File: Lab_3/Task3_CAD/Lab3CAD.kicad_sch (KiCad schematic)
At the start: 25 parts, among them J1 Conn_01x02, T1 Transformer_1P_1S, T2 Transformer_1P_1S, U1 LM317_TO-220, U2 LM337_TO220

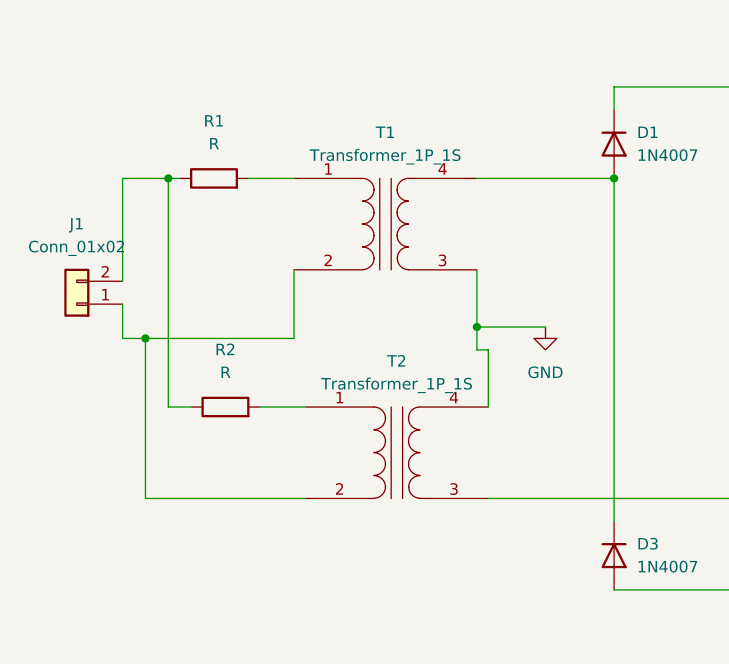
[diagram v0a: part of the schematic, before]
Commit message: block diagram
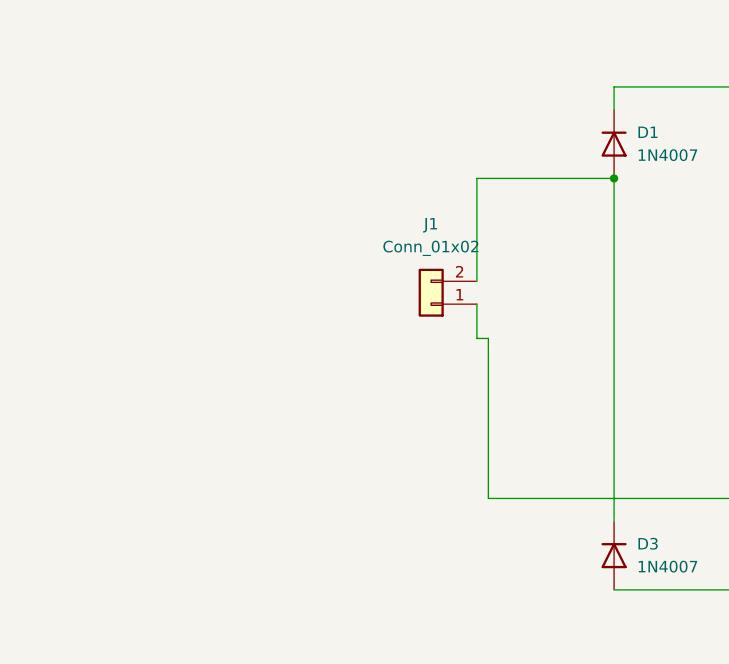
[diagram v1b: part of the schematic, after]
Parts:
- removed R1, R2: R, Resistor_THT:R_Axial_DIN0207_L6.3mm_D2.5mm_P7.62mm_Horizontal, symbol Device:R
- removed T1, T2: Transformer_1P_1S, Transformer_THT:Transformer_Zeming_ZMPT101K, symbol Device:Transformer_1P_1S
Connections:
- net at J1.2 (Pin_2): now also D1.2 (A), D3.1 (K)
- net at D2.2 (A), D4.1 (K): now also J1.1 (Pin_1)
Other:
- moved on the sheet: J1
